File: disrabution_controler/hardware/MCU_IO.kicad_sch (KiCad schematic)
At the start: 48 parts, among them J1 Conn_Coaxial, J2 PROG_PORT, J3 JTAG, Q17 NMOS, U2 ESP32-S2FH2, U3 ECMF02-2AMX6, U9 PI4IOE5V6416LEX, Y1 40 MHz

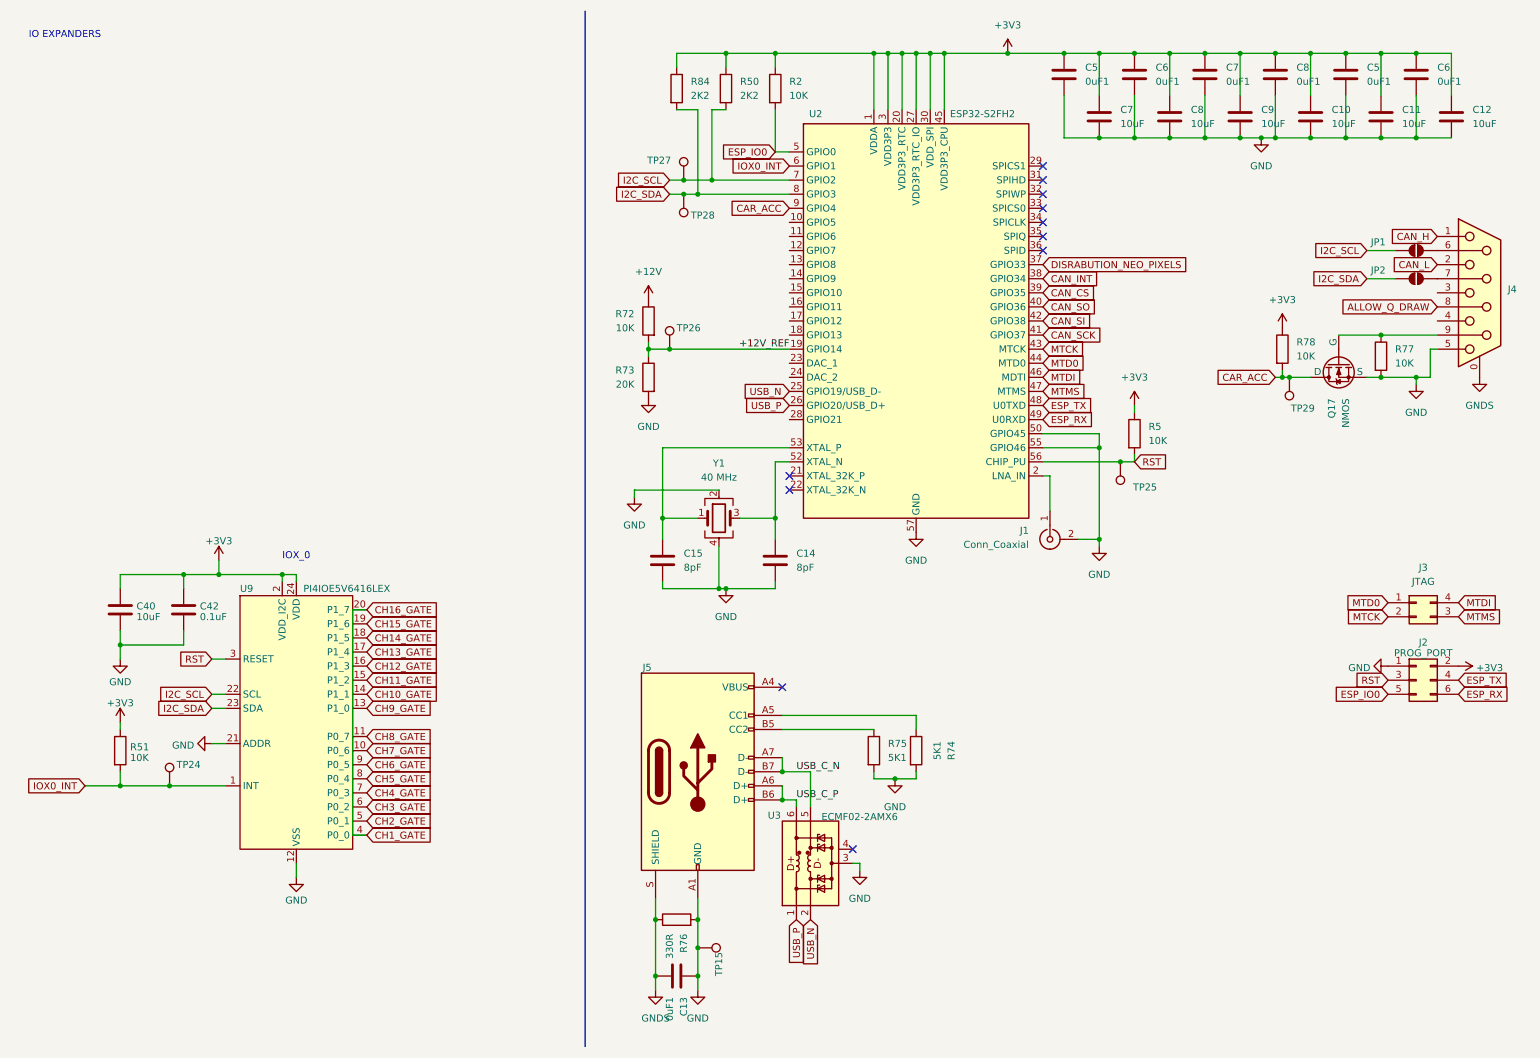
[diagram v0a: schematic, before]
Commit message: more hardware work
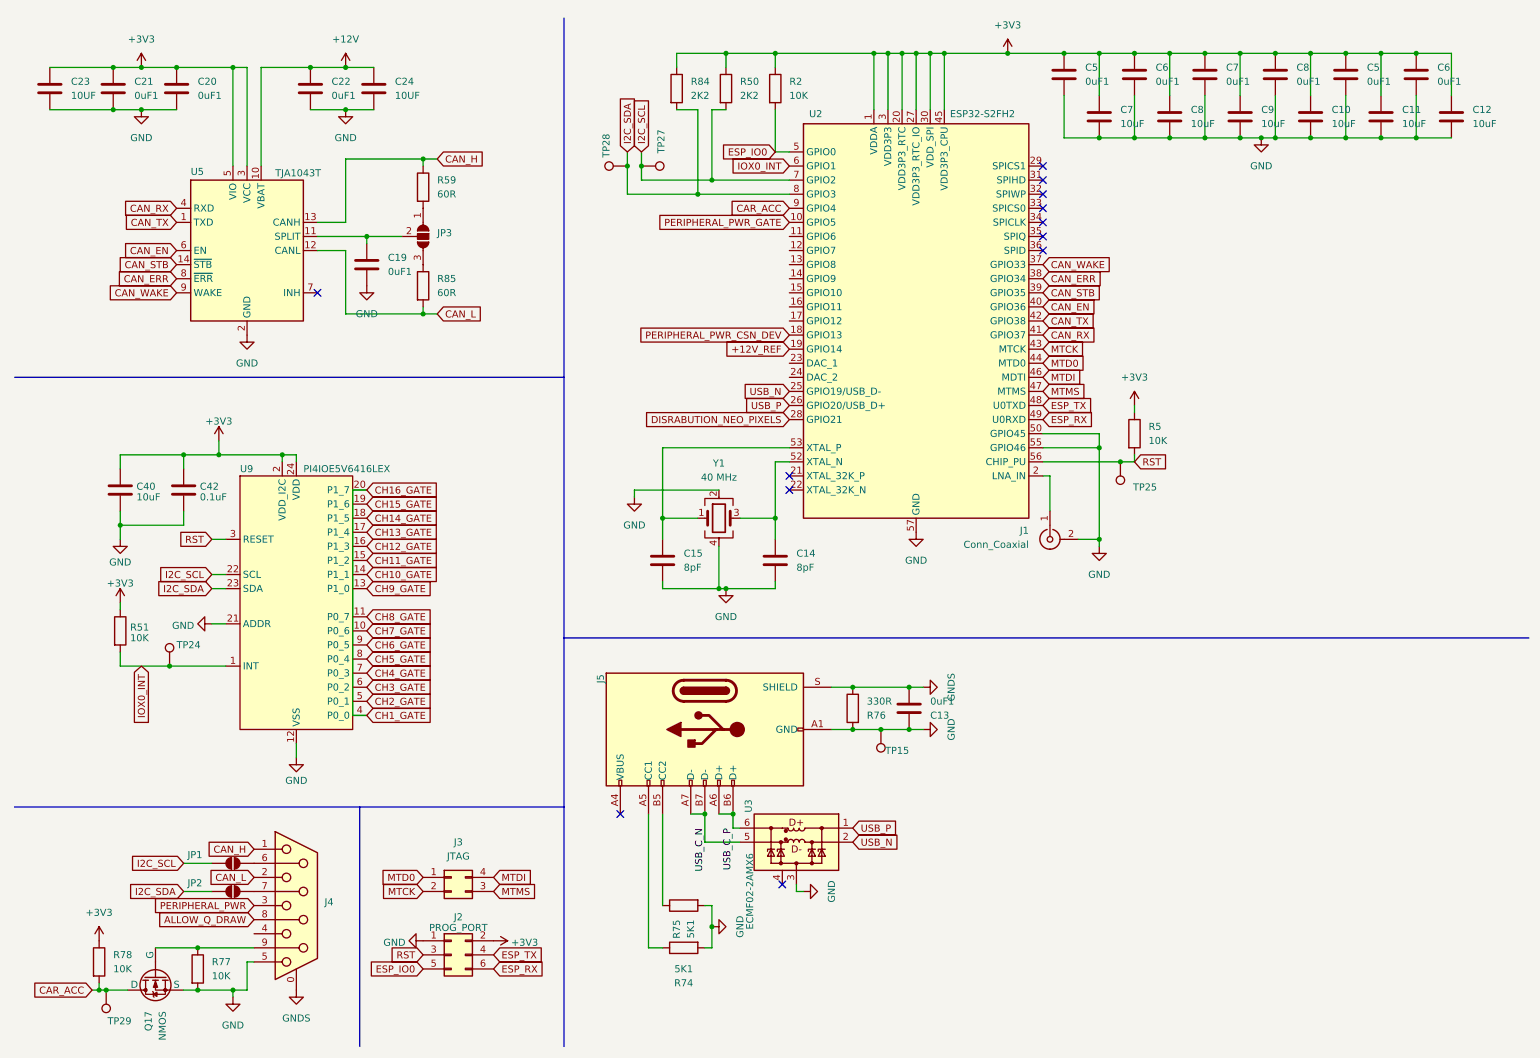
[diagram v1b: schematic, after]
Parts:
- removed R72: 10K, symbol Device:R
- removed R73: 20K, symbol Device:R
- removed TP26: ~, symbol Connector:TestPoint
- added C19, C20, C21, C22: 0uF1, symbol Device:C
- added C23, C24: 10UF, symbol Device:C
- added JP3: ~, symbol Jumper:SolderJumper_3_Open
- added R59, R85: 60R, symbol Device:R
- added U5: TJA1043T, Package_SO:SOIC-14_3.9x8.7mm_P1.27mm, symbol Interface_CAN_LIN:TJA1043T
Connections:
- net +12V: now also C22.1, C24.1, U5.10 (VBAT)
- net +3V3: now also C20.1, C21.1, C23.1, U5.3 (VCC), U5.5 (VIO)
- net CAN_H: now also R59.1, U5.13 (CANH)
- net CAN_L: now also R85.2, U5.12 (CANL)
- net DISRABUTION_NEO_PIXELS: now also U2.28 (GPIO21); no longer U2.37 (GPIO33)
- net GND: now also C19.2, C20.2, C21.2, C22.2, C23.2, C24.2, U5.2 (GND)
- net PERIPHERAL_PWR: now reaches J4.3
- net PERIPHERAL_PWR_GATE: now reaches U2.10 (GPIO5)
- net PERIPHERAL_PWR_CSN_DEV: now reaches U2.18 (GPIO13)
- net CAN_CS renamed CAN_STB
- net CAN_STB: now also U5.14 (~{STB})
- net CAN_INT renamed CAN_ERR
- net CAN_ERR: now also U5.8 (~{ERR})
- net CAN_SCK renamed CAN_RX
- net CAN_RX: now also U5.4 (RXD)
- net CAN_SI renamed CAN_TX
- net CAN_TX: now also U5.1 (TXD)
- net CAN_SO renamed CAN_EN
- net CAN_EN: now also U5.6 (EN)
- new net: JP3.1 (A), R59.2
- new net: C19.1, JP3.2 (C), U5.11 (SPLIT)
- new net: JP3.3 (B), R85.1
- new net CAN_WAKE: U2.37 (GPIO33), U5.9 (WAKE)
- no-connect marks 11 -> 12
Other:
- note removed: "IO EXPANDERS"
- note removed: "IOX_0"
- moved on the sheet: C13, C40, C42, J2, J3, J4, J5, JP1, JP2, Q17, R51, R74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
